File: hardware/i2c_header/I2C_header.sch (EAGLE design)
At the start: 5 parts

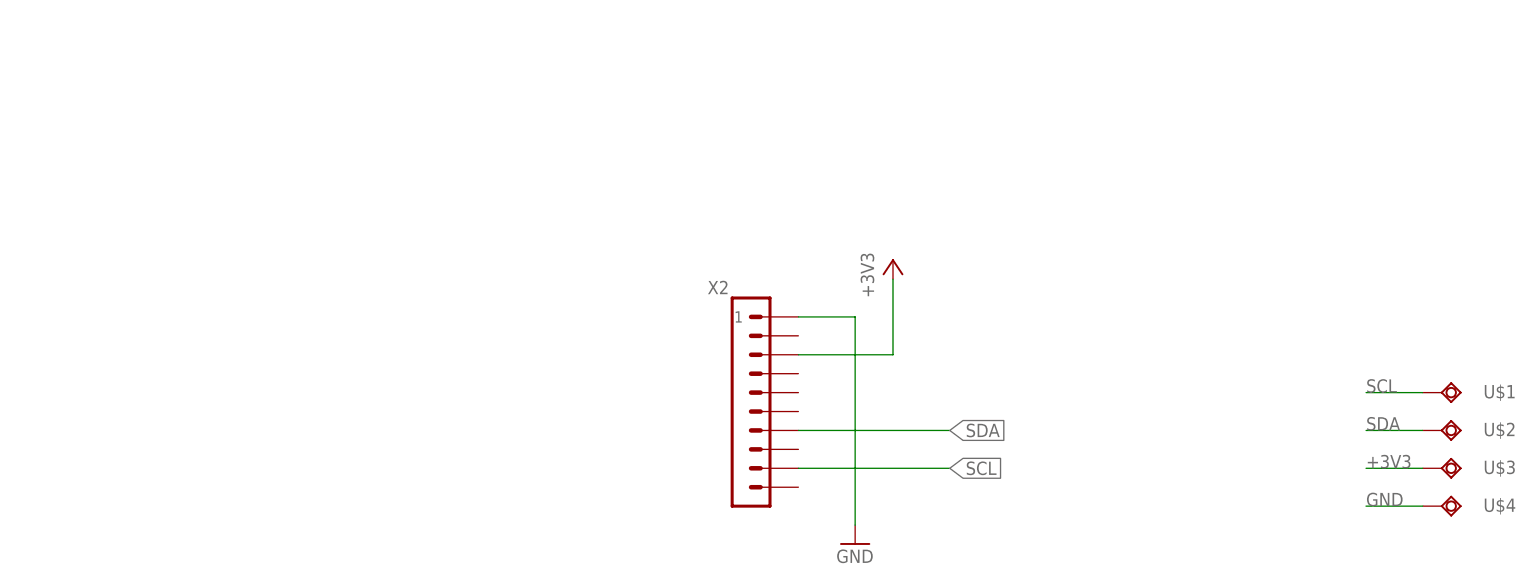
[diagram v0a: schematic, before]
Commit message: Latest hardware designs
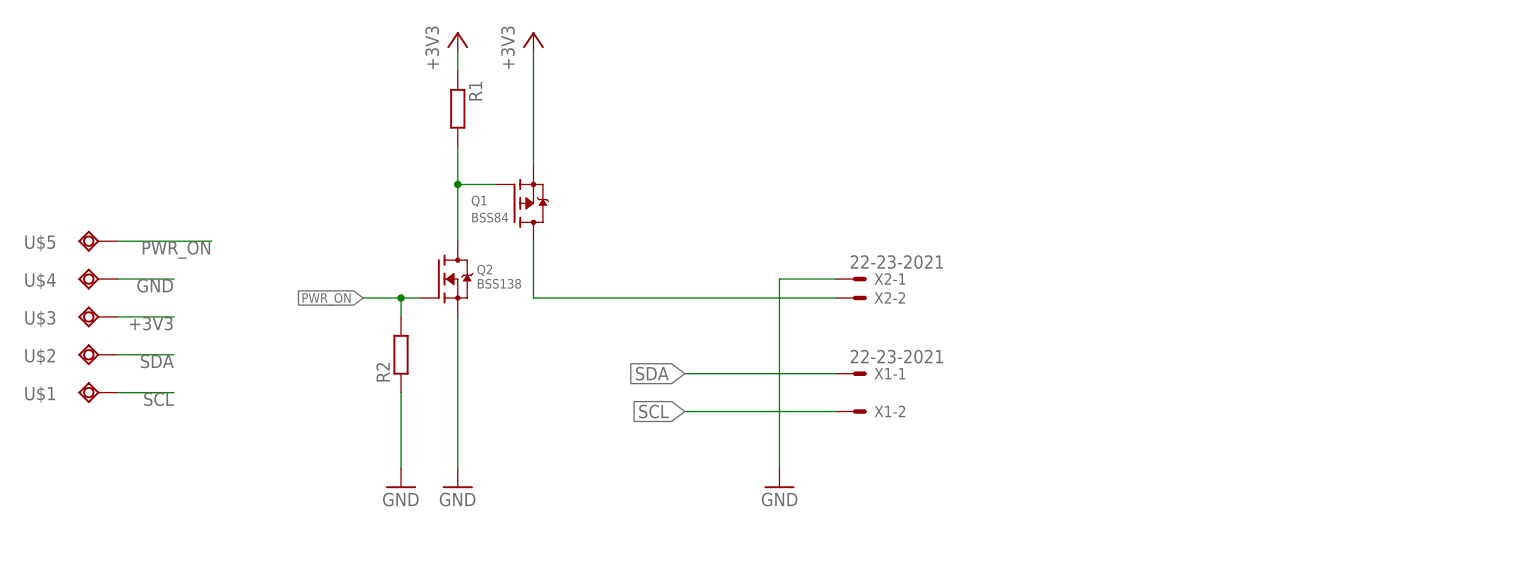
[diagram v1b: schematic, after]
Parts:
- added Q1: BSS84, SIG_Parts:BSS84
- added Q2: BSS138, SIG_Parts:BSS138
- added R1, R2: (no value), SIG_Parts:RESISTOR_0805
- added U$5: PAD3.0X5.0, SIG_Parts:PAD3.0X5.0
- added X1: 22-23-2021, con-molex:22-23-2021
- X2: value (none) -> 22-23-2021; device SIG_Parts:FFC_10PLARGE -> con-molex:22-23-2021
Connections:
- new net N$1: Q1.D, X2-2.S
- new net N$2: Q1.G, Q2.D, R1.2
- new net PWR_ON: Q2.G, R2.2, U$5.P$1
- net +3V3: now also Q1.S, R1.1; no longer X2G$1.3
- net GND: now also Q2.S, R2.1, X2-1.S; no longer X2G$1.1
- net SCL: now also X1-2.S; no longer X2G$1.9
- net SDA: now also X1-1.S; no longer X2G$1.7
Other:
- moved on the sheet: U$1, U$2, U$3, U$4
